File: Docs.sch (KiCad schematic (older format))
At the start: 0 parts

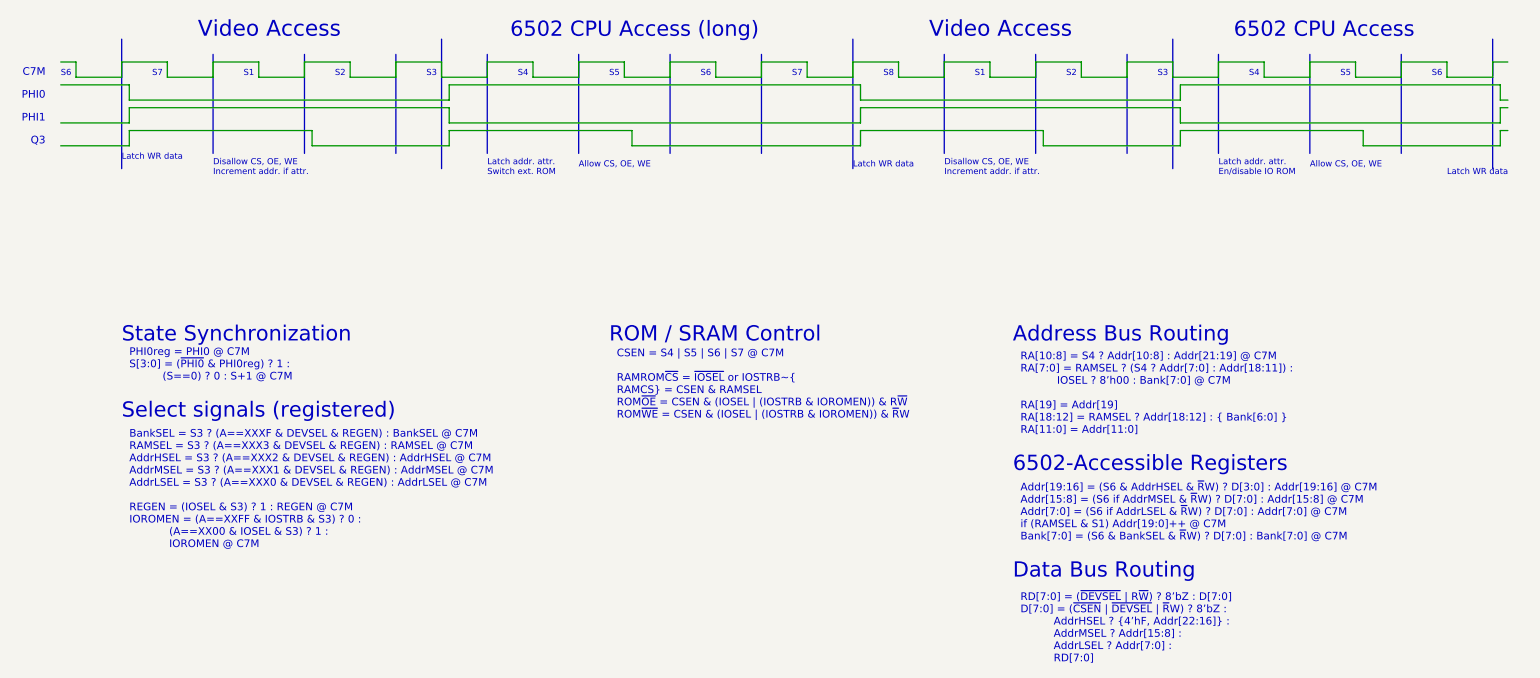
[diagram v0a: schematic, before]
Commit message: Can't fit...
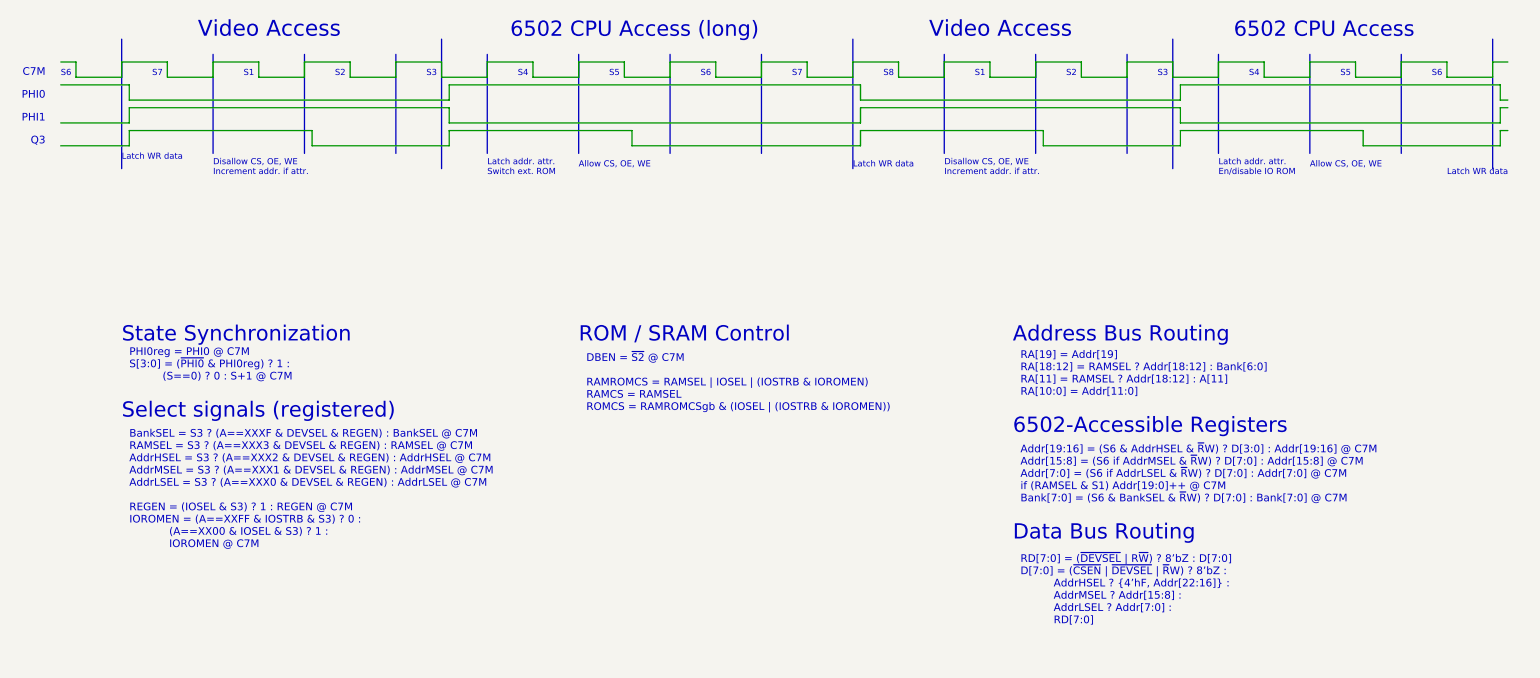
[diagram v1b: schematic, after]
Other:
- note added: "DBEN = ~S2~ @ C7M\n\nRAMROMCS = RAMSEL | IOSEL | (IOSTRB & IOROMEN)\nRAMCS = RAMSEL\nROMCS = RAMROMCSgb & (IOSEL | (IOSTRB & IOROMEN))"
- note added: "RA[19] = Addr[19]\nRA[18:12] = RAMSEL ? Addr[18:12] : Bank[6:0]\nRA[11] = RAMSEL ? Addr[18:12] : A[11]\nRA[10:0] = Addr[11:0]"
- note removed: "CSEN = S4 | S5 | S6 | S7 @ C7M\n\nRAMROM~CS~ = ~IOSEL or IOSTRB~\nRAMCS = CSEN & RAMSEL\nROM~OE~ = CSEN & (IOSEL | (IOSTRB & IOROMEN)) & R~W~\nROM~WE~ = CSEN & (IOSEL | (IOSTRB & IOROMEN)) & ~R~W"
- note removed: "RA[10:8] = S4 ? Addr[10:8] : Addr[21:19] @ C7M\nRA[7:0] = RAMSEL ? (S4 ? Addr[7:0] : Addr[18:11]) : \n IOSEL ? 8’h00 : Bank[7:0] @ C7M\n\nRA[19] = Addr[19]\nRA[18:12] = RAMSEL ? Addr[18:12] : { Bank[6:0] }\nRA[11:0] = Addr[11:0]"
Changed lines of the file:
@@
 Wire Wire Line
 	5200 1000 5200 1100
-Text Notes 4550 3350 0    50   ~ 0
-CSEN = S4 | S5 | S6 | S7 @ C7M\n\nRAMROM~CS~ = ~IOSEL or IOSTRB~\nRAMCS = CSEN & RAMSEL\nROM~OE~ = CSEN & (IOSEL | (IOSTRB & IOROMEN)) & R~W~\nROM~WE~ = CSEN & (IOSEL | (IOSTRB & IOROMEN)) & ~R~W
 Text Notes 1350 3100 0    50   ~ 0
 PHI0reg = PHI0 @ C7M\nS[3:0] = (~PHI0~ & PHI0reg) ? 1 : \n          (S==0) ? 0 : S+1 @ C7M
@@
 Text Notes 1300 2850 0    100  ~ 0
 State Synchronization
-Text Notes 4500 2850 0    100  ~ 0
+Text Notes 4300 2850 0    100  ~ 0
 ROM / SRAM Control
 Text Notes 1350 4200 0    50   ~ 0
@@
 Text Notes 7150 2850 0    100  ~ 0
 Address Bus Routing
-Text Notes 7150 3700 0    100  ~ 0
-6502-Accessible Registers
-Text Notes 7150 4400 0    100  ~ 0
-Data Bus Routing
-Text Notes 7200 4950 0    50   ~ 0
-RD[7:0] = (~DEVSEL~ | R~W~) ? 8’bZ : D[7:0]\nD[7:0] = (~CSEN~ | ~DEVSEL~ | ~R~W) ? 8’bZ :\n          AddrHSEL ? {4’hF, Addr[22:16]} : \n          AddrMSEL ? Addr[15:8] : \n          AddrLSEL ? Addr[7:0] :\n          RD[7:0]
 Wire Wire Line
 	10300 1000 10400 1000
@@
 Wire Wire Line
 	10350 1450 10400 1450
-Text Notes 7200 3450 0    50   ~ 0
-RA[10:8] = S4 ? Addr[10:8] : Addr[21:19] @ C7M\nRA[7:0] = RAMSEL ? (S4 ? Addr[7:0] : Addr[18:11]) : \n           IOSEL ? 8’h00 : Bank[7:0] @ C7M\n\nRA[19] = Addr[19]\nRA[18:12] = RAMSEL ? Addr[18:12] : { Bank[6:0] }\nRA[11:0] = Addr[11:0]
-Text Notes 7200 4150 0    50   ~ 0
-Addr[19:16] = (S6 & AddrHSEL & ~R~W) ? D[3:0] : Addr[19:16] @ C7M\nAddr[15:8] = (S6 if AddrMSEL & ~R~W) ? D[7:0] : Addr[15:8] @ C7M\nAddr[7:0] = (S6 if AddrLSEL & ~R~W) ? D[7:0] : Addr[7:0] @ C7M\nif (RAMSEL & S1) Addr[19:0]++ @ C7M\nBank[7:0] = (S6 & BankSEL & ~R~W) ? D[7:0] : Bank[7:0] @ C7M
+Text Notes 7200 3200 0    50   ~ 0
+RA[19] = Addr[19]\nRA[18:12] = RAMSEL ? Addr[18:12] : Bank[6:0]\nRA[11] = RAMSEL ? Addr[18:12] : A[11]\nRA[10:0] = Addr[11:0]
 Text Notes 10000 1750 0    40   ~ 0
 Latch WR data
@@
 Text Notes 8500 1750 0    40   ~ 0
 Latch addr. attr.\nEn/disable IO ROM
+Text Notes 7150 3450 0    100  ~ 0
+6502-Accessible Registers
+Text Notes 7150 4150 0    100  ~ 0
+Data Bus Routing
+Text Notes 7200 4700 0    50   ~ 0
+RD[7:0] = (~DEVSEL~ | R~W~) ? 8’bZ : D[7:0]\nD[7:0] = (~CSEN~ | ~DEVSEL~ | ~R~W) ? 8’bZ :\n          AddrHSEL ? {4’hF, Addr[22:16]} : \n          AddrMSEL ? Addr[15:8] : \n          AddrLSEL ? Addr[7:0] :\n          RD[7:0]
+Text Notes 7200 3900 0    50   ~ 0
+Addr[19:16] = (S6 & AddrHSEL & ~R~W) ? D[3:0] : Addr[19:16] @ C7M\nAddr[15:8] = (S6 if AddrMSEL & ~R~W) ? D[7:0] : Addr[15:8] @ C7M\nAddr[7:0] = (S6 if AddrLSEL & ~R~W) ? D[7:0] : Addr[7:0] @ C7M\nif (RAMSEL & S1) Addr[19:0]++ @ C7M\nBank[7:0] = (S6 & BankSEL & ~R~W) ? D[7:0] : Bank[7:0] @ C7M
+Text Notes 4350 3300 0    50   ~ 0
+DBEN = ~S2~ @ C7M\n\nRAMROMCS = RAMSEL | IOSEL | (IOSTRB & IOROMEN)\nRAMCS = RAMSEL\nROMCS = RAMROMCSgb & (IOSEL | (IOSTRB & IOROMEN))
 $EndSCHEMATC
